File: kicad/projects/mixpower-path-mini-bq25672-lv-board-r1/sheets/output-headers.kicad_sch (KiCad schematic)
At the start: 8 parts, among them J5 PWR_HEADER, J6 DATA_CONN, J7 DATA_HEADER, J8 HAT, J9 DEBUG

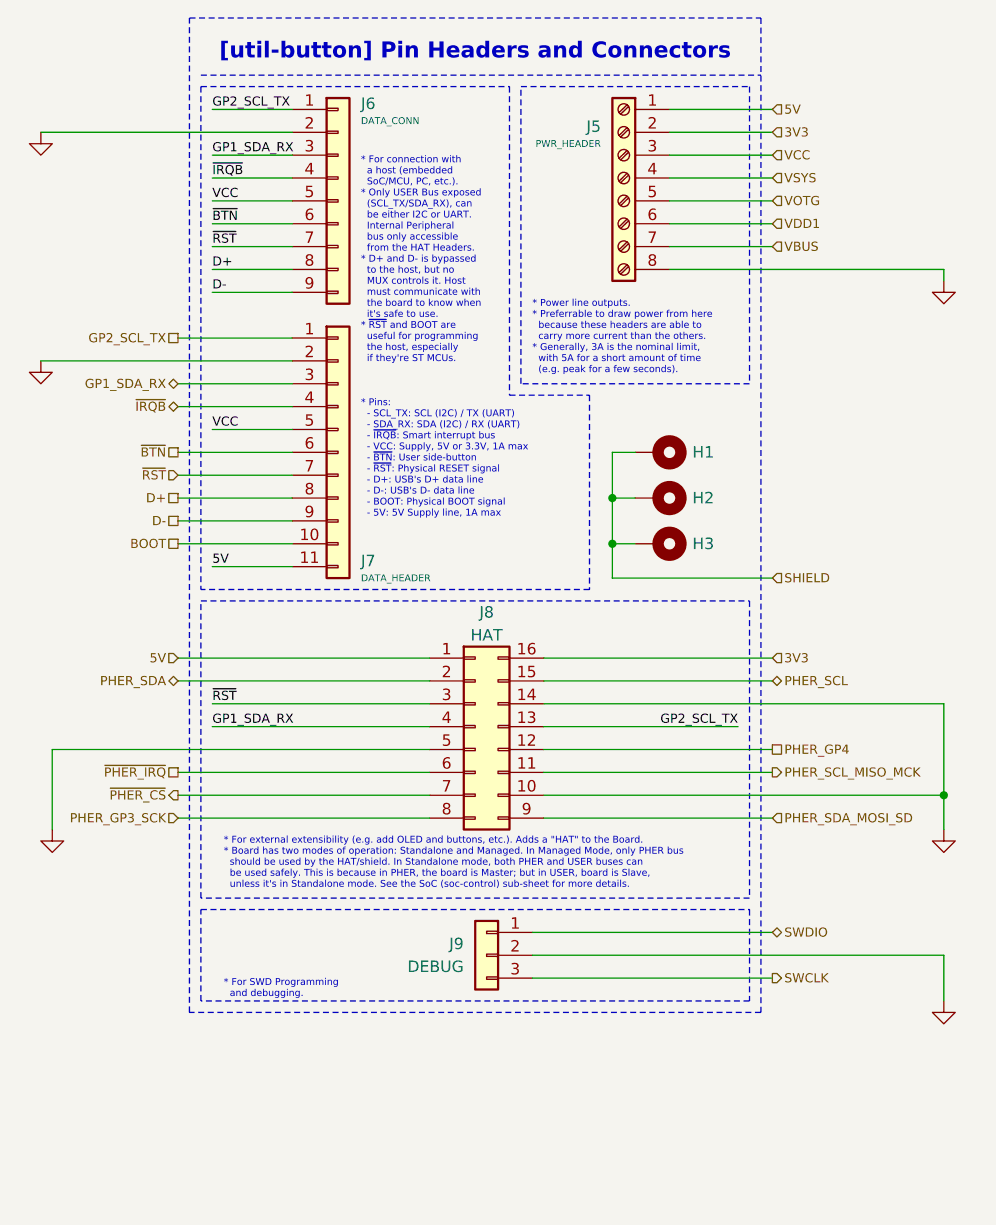
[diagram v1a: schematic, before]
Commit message: feat: failed PCB routing
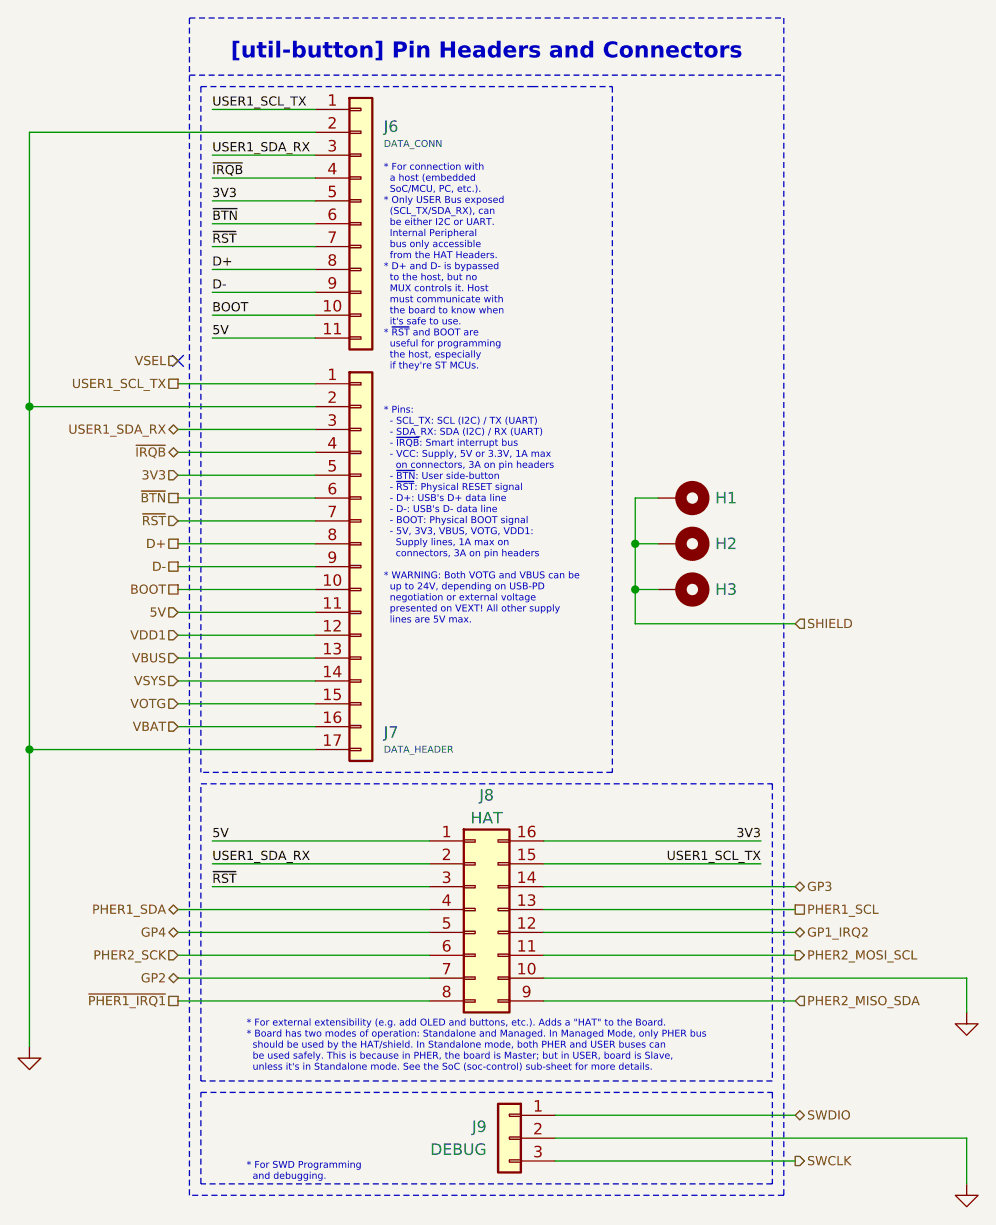
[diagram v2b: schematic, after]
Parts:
- removed J5: PWR_HEADER, Connector_PinHeader_2.54mm:PinHeader_1x08_P2.54mm_Vertical, symbol Connector:Screw_Terminal_01x08
- J6: footprint Connector_JST:JST_ZH_B9B-ZR_1x09_P1.50mm_Vertical -> Connector_Molex:Molex_PicoBlade_53047-1110_1x11_P1.25mm_Vertical; symbol Connector_Generic:Conn_01x09 -> Connector_Generic:Conn_01x11
- J7: footprint Connector_PinHeader_2.54mm:PinHeader_1x11_P2.54mm_Vertical -> Connector_PinHeader_2.54mm:PinHeader_1x17_P2.54mm_Vertical; symbol Connector_Generic:Conn_01x11 -> Connector_Generic:Conn_01x17
- J8: footprint Connector_IDC:IDC-Header_2x08_P2.54mm_Vertical -> Connector_JST:JST_PHD_B16B-PHDSS_2x08_P2.00mm_Vertical
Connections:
- net PHER_SCL is gone; now on net USER1_SCL_TX: J8.15 (Pin_15)
- net PHER_SDA is gone; now on net USER1_SDA_RX: J8.2 (Pin_2)
- net VCC is gone; now on net 3V3: J6.5 (Pin_5), J7.5 (Pin_5)
- net 5V: now also J6.11 (Pin_11)
- net BOOT: now also J6.10 (Pin_10)
- net GND: now also J7.17 (Pin_17); no longer J8.14 (Pin_14), J8.5 (Pin_5)
- net VBUS: now also J7.13 (Pin_13)
- net VDD1: now also J7.12 (Pin_12)
- net VOTG: now also J7.15 (Pin_15)
- net VSYS: now also J7.14 (Pin_14)
- net GP1_SDA_RX renamed USER1_SDA_RX
- net USER1_SDA_RX: no longer J8.4 (Pin_4)
- net GP2_SCL_TX renamed USER1_SCL_TX
- net USER1_SCL_TX: no longer J8.13 (Pin_13)
- net PHER_GP3_SCK renamed ~{PHER1_IRQ1}
- net PHER_GP4 renamed GP1_IRQ2
- net PHER_SCL_MISO_MCK renamed PHER2_MOSI_SCL
- net PHER_SDA_MOSI_SD renamed PHER2_MISO_SDA
- net ~{PHER_CS} renamed GP2
- net ~{PHER_IRQ} renamed PHER2_SCK
- new net GP3: J8.14 (Pin_14)
- new net GP4: J8.5 (Pin_5)
- new net PHER1_SCL: J8.13 (Pin_13)
- new net PHER1_SDA: J8.4 (Pin_4)
- new net VBAT: J7.16 (Pin_16)
- no-connect marks 0 -> 1
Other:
- note removed: "* Power line outputs. * Preferrable to draw power from here because these headers are able to carry more current than the others. * Generally, 3A is the nominal limit, with 5A for a short amount of time (e.g. peak for a few seconds)."
- moved on the sheet: H1, H2, H3, J8, J9
